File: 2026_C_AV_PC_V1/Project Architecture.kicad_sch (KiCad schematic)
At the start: 0 parts

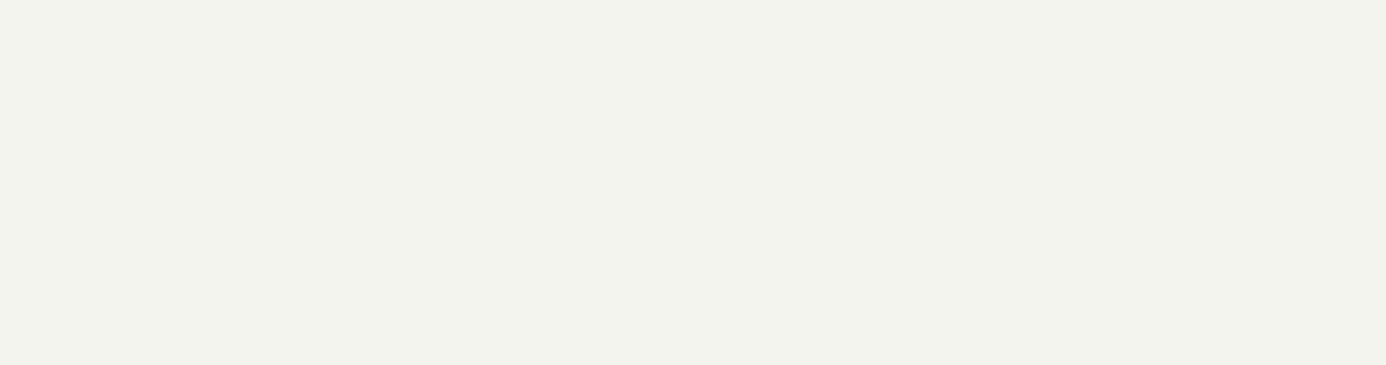
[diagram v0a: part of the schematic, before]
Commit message: spine almost finished
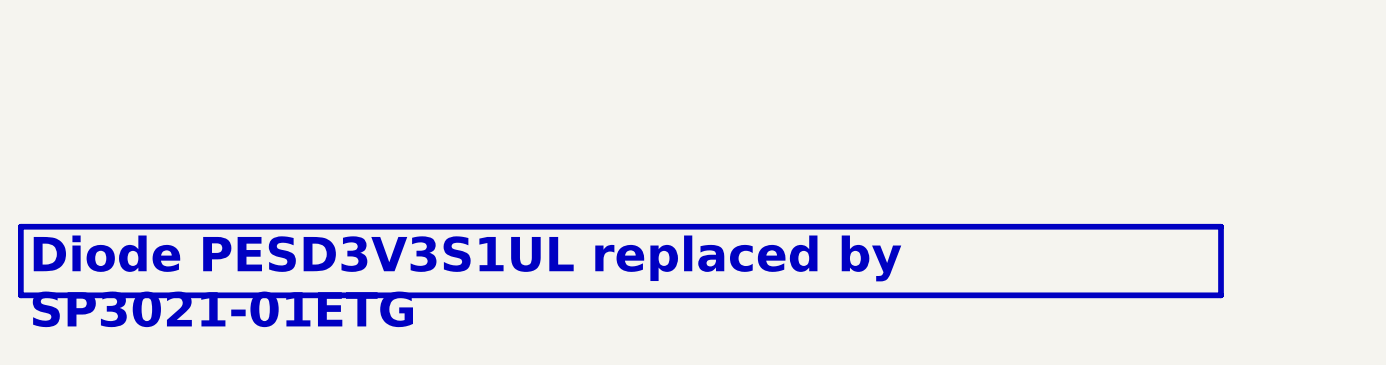
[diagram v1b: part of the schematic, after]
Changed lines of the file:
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@@
+		)
+	)
+	(text_box "Diode PESD3V3S1UL replaced by SP3021-01ETG"
+		(exclude_from_sim no)
+		(at 12.7 189.23 0)
+		(size 133.35 7.62)
+		(margins 0.9525 0.9525 0.9525 0.9525)
+		(stroke
+			(width 0.635)
+			(type solid)
+			(color 255 0 0 1)
+		)
+		(fill
+			(type none)
+		)
+		(effects
+			(font
+				(face "SF Pro Text")
+				(size 3.81 3.81)
+				(bold yes)
+				(color 255 0 0 1)
+			)
+			(justify left top)
 		)
 	)
